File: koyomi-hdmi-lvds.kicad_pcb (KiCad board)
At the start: 2 copper layers, 89.1 x 37.5 mm, 42 parts, among them IC1 SN75LVDS83B, J1 20374-R30E-31, J2 HDMI_I2C, J3 I/O, U1 TFP401, U2 24LC02B, U3 AP2114H-2.5

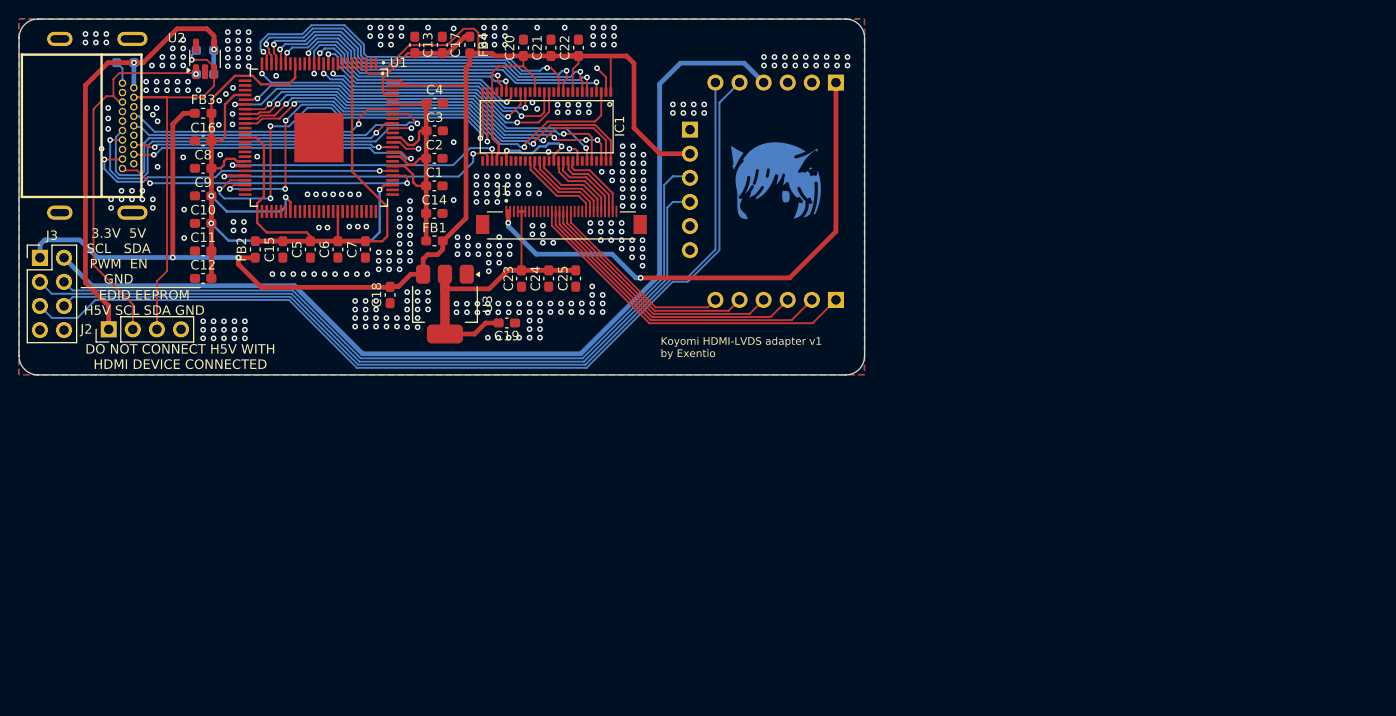
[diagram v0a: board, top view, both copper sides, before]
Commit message: Rerouting by @CRImier
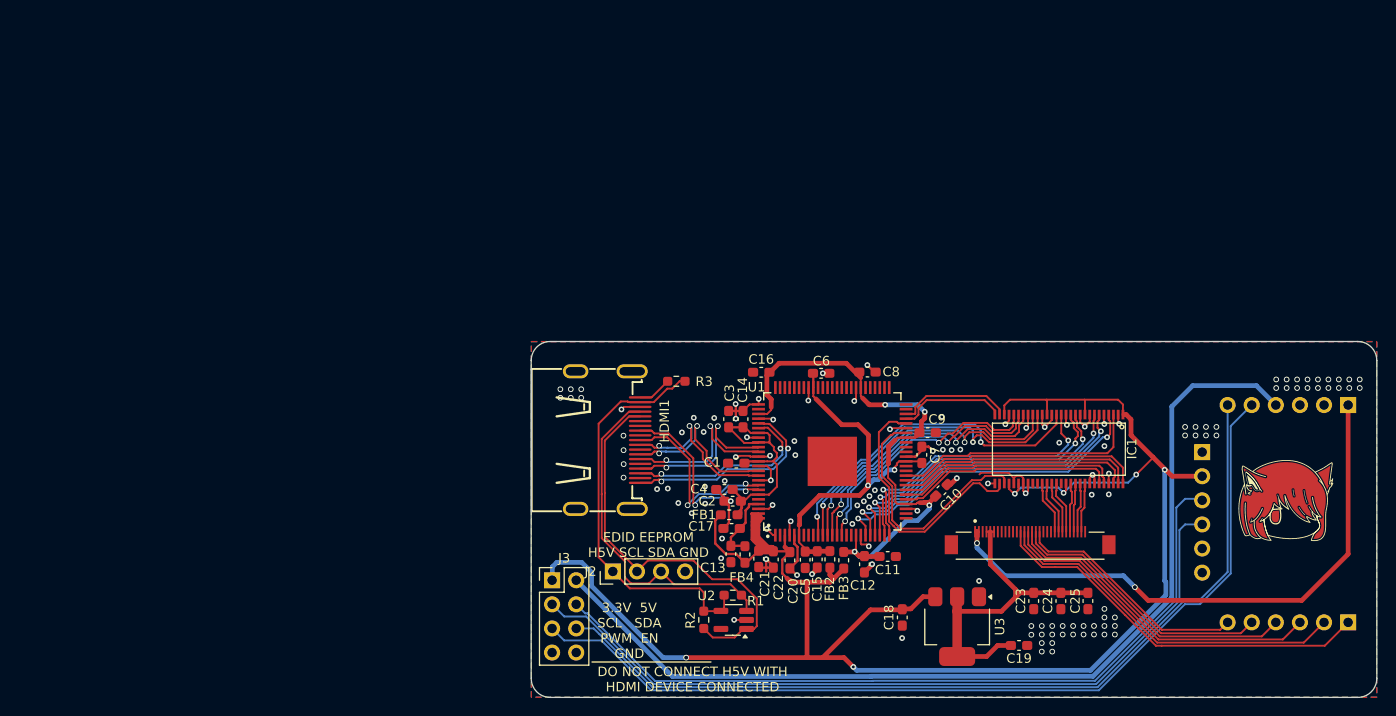
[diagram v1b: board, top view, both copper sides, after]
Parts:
- HDMI1: value U-C-19DD-W-1 -> HDMI-019S; footprint U-C-19DD-W-1:U-C-19DD-W-1 -> HDMI_SMD:HDMI-SMD_HDMI-019S
- J4: value (none) -> ~
- R1, R2, R3, REF**: moved to F.Cu
- moved C10 82.7 mm to (109.3, 61.9), turned to 45 degrees
- moved FB3 82.3 mm to (99.0, 69.2), turned to 90 degrees
- moved U2 81.2 mm to (87.4, 75.5), turned to 180 degrees
- moved C9 80.3 mm to (107.8, 55.8), turned to 0 degrees
- moved R1 79.9 mm to (87.3, 72.9), turned to 0 degrees
- moved C11 79.0 mm to (103.6, 68.8), turned to 0 degrees
- moved R2 77.9 mm to (84.2, 75.5), turned to -90 degrees
- moved C12 75.9 mm to (101.2, 69.7), turned to -90 degrees
- moved C8 73.2 mm to (101.5, 49.4), turned to 0 degrees
- moved FB2 68.8 mm to (97.5, 69.1)
- moved R3 67.1 mm to (81.4, 50.4)
- moved C15 65.1 mm to (96.2, 69.1)
- moved U1 64.0 mm to (97.8, 58.8), turned to 90 degrees
- moved C18 63.8 mm to (105.2, 75.3)
- moved C19 63.8 mm to (117.5, 78.2)
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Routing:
- net GND: track 7.90 -> 79.3 mm, vias 373 -> 129
- net VSYNC: track 46.3 -> 11.4 mm, vias 4 -> 0
- net HSYNC: track 43.9 -> 12.2 mm, vias 4 -> 0
- net TX0+: track 42.4 -> 18.2 mm
- net R1: track 44.0 -> 23.7 mm, vias 2 -> 0
- net TX0-: track 37.9 -> 18.2 mm, vias 1 -> 2
- net OVDD: track 79.1 -> 59.7 mm
- net R4: track 45.2 -> 26.1 mm, vias 2 -> 0
- net R3: track 44.1 -> 25.5 mm, vias 2 -> 0
- net R5: track 44.5 -> 26.5 mm, vias 2 -> 0
- net +3V3: track 183.8 -> 201.5 mm, vias 4 -> 6
- net R0: track 40.7 -> 23.0 mm, vias 2 -> 0
- net R2: track 42.4 -> 25.0 mm, vias 4 -> 0
- net DVDD: track 54.4 -> 37.7 mm, vias 0 -> 2
- net TXC+: track 33.7 -> 19.7 mm, vias 1 -> 2
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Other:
- board text removed: "Koyomi HDMI-LVDS adapter v1 by Exentio"
